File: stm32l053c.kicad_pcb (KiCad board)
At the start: 2 copper layers, 20.8 x 43.7 mm, 17 parts, among them P1 SWD, P2 CONN_01X17, P3 CONN_01X17, P4 Ext Xtal, SW1 RESET, U1 STM32L053C8_LQFP48

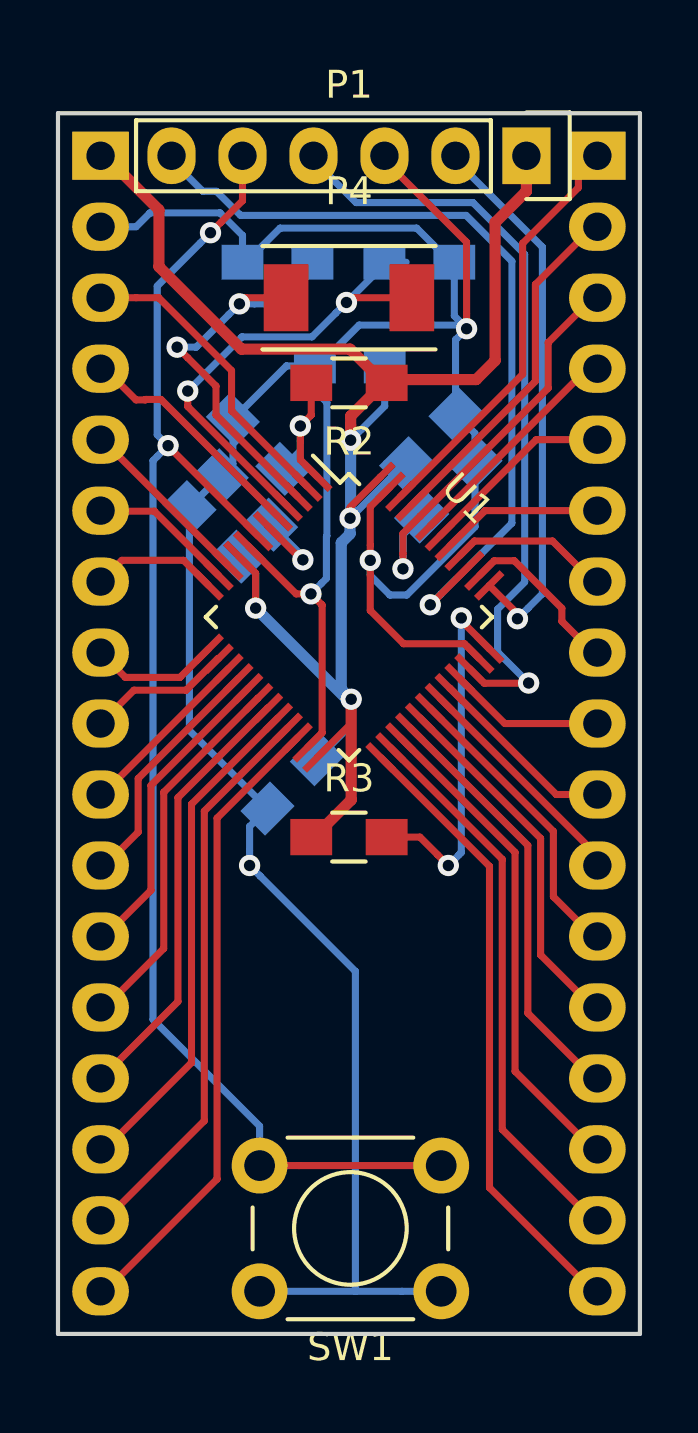
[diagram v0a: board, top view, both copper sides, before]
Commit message: Solder bridges
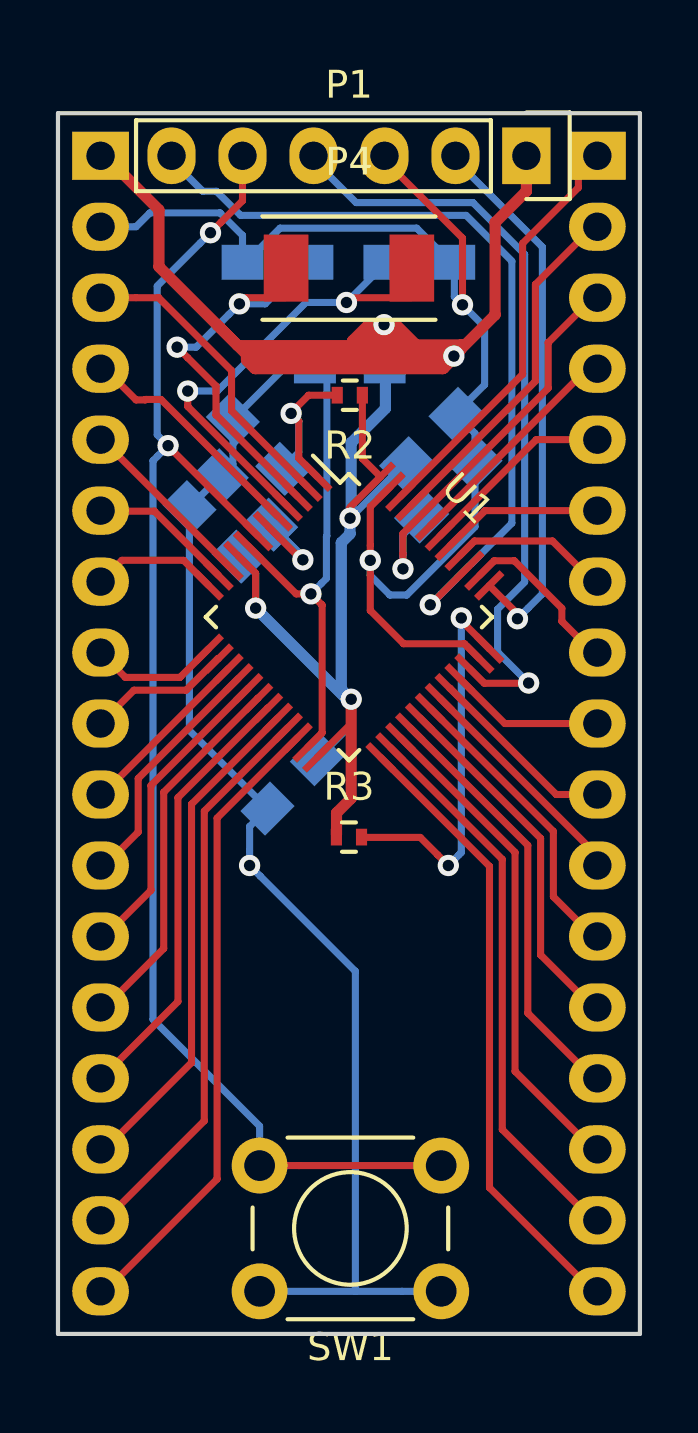
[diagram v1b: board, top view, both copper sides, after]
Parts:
- R2, R3: footprint Resistors_SMD:R_0805_HandSoldering -> Resistors_SMD:R_0402
- moved P4 1.06 mm to (191.8, 85.3)
- moved R2 0.44 mm to (191.8, 89.8)
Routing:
- net VDD: track 66.7 -> 93.6 mm, vias 4 -> 5
- net Earth: track 116.3 -> 109.4 mm
- net /VLCD: track 5.58 -> 6.88 mm
- net /VDD_USB: track 13.2 -> 14.1 mm

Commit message: Extra ground
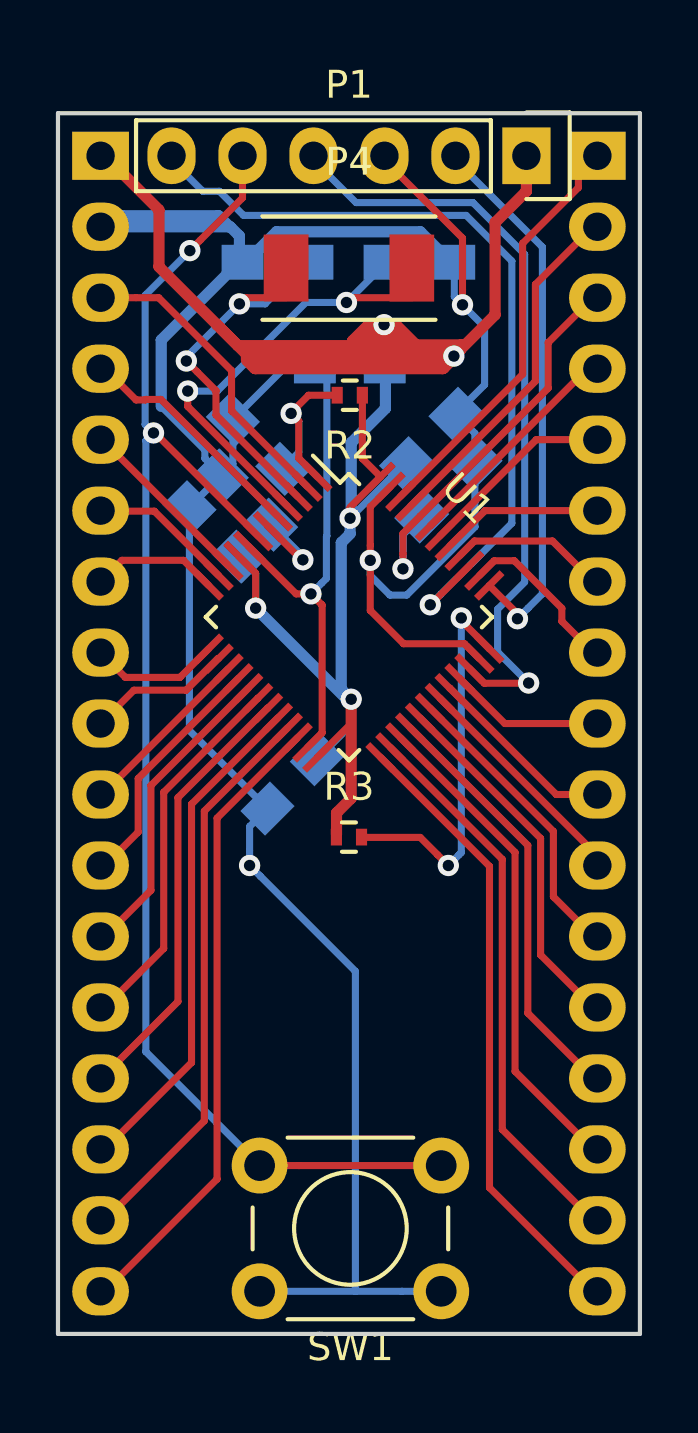
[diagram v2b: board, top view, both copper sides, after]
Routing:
- net Earth: track 109.4 -> 122.7 mm
- net NRST: track 50.4 -> 51.3 mm
- net OSC32_OUT: track 17.8 -> 17.0 mm
- net OSC32_IN: track 15.0 -> 14.3 mm
